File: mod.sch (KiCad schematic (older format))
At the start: 17 parts, among them IC1 ATTINY85-S, J1 MICROUSB, P1 CONN_12, Q2 FDD8870, SW1 SW_PUSH_SMALL, SW2 SW_PUSH_SMALL, SW3 SW_PUSH_SMALL

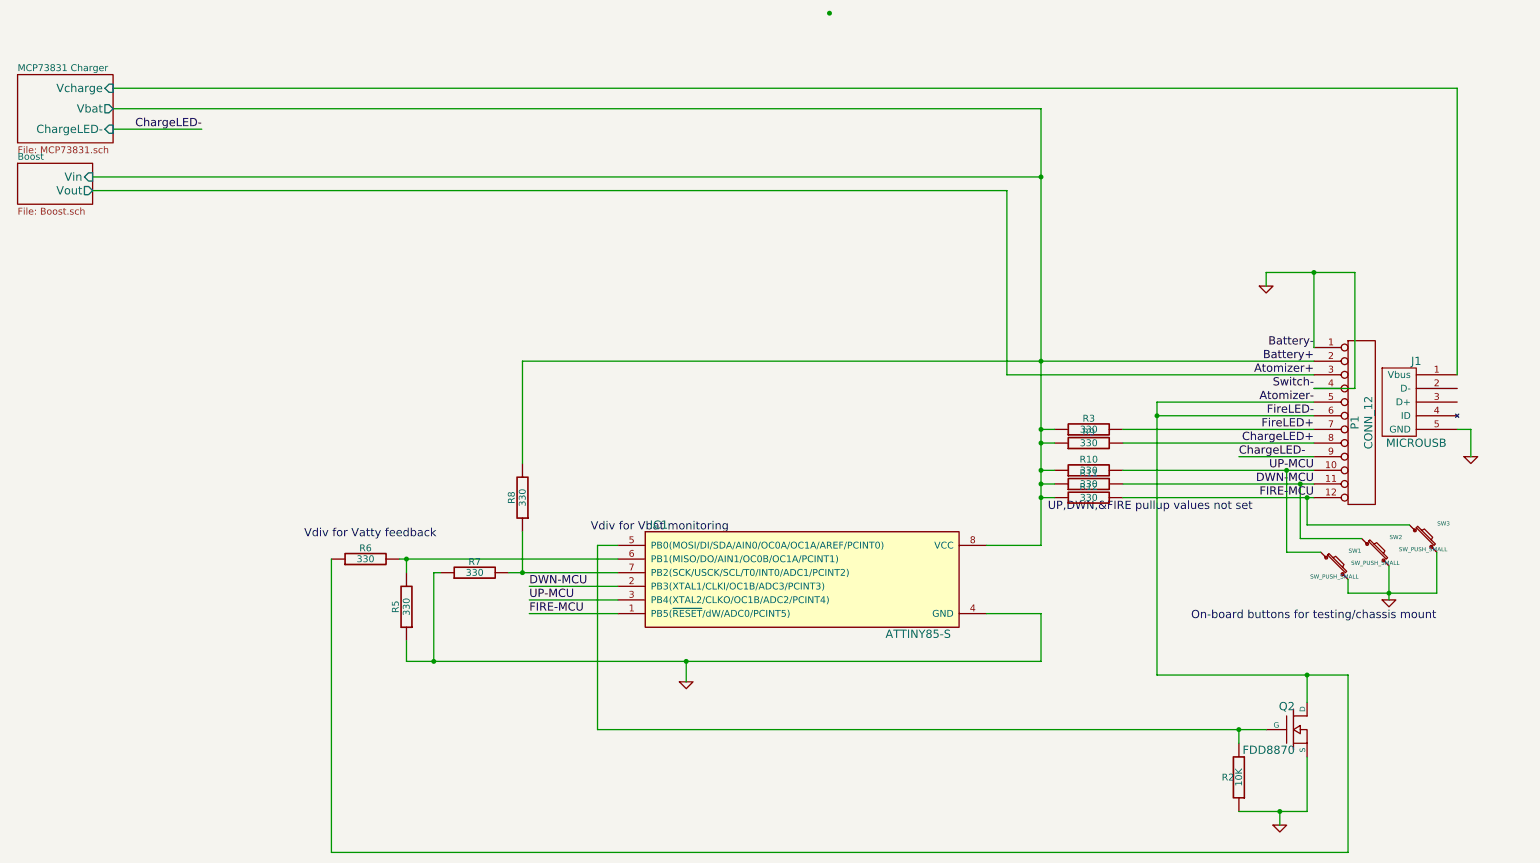
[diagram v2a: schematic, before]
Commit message: many changes. Most not stable. Check TODO
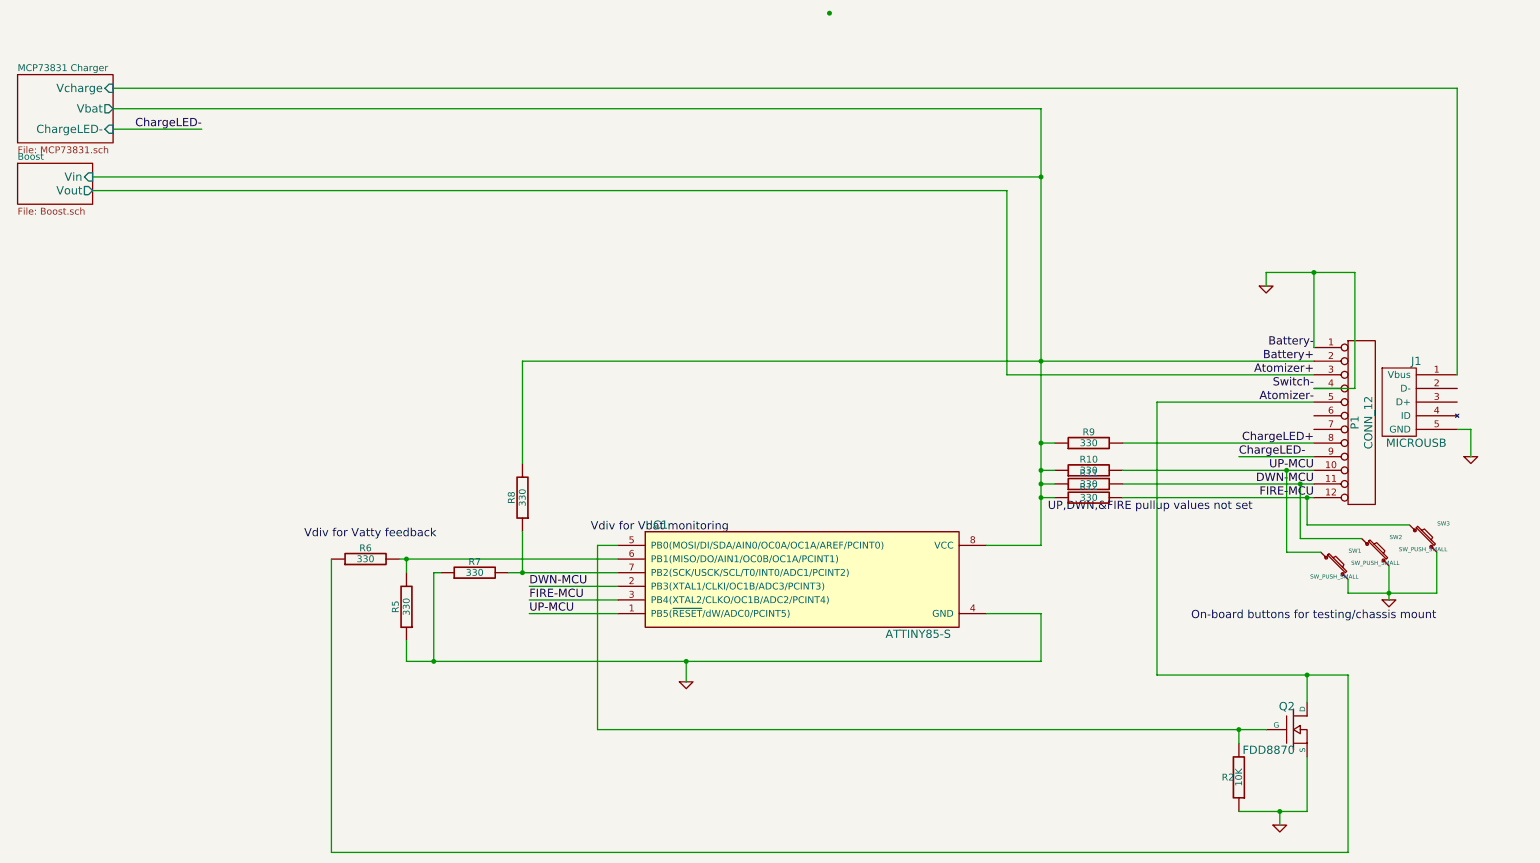
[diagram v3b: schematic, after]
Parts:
- removed R3: 330, symbol R
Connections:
- net Atomizer-: no longer P1.6 (P6)
- net FIRE-MCU: now also IC1.3 (PB4(XTAL2/CLKO/OC1B/ADC2/PCINT4)); no longer IC1.1 (PB5(~RESET~/dW/ADC0/PCINT5))
- net UP-MCU: now also IC1.1 (PB5(~RESET~/dW/ADC0/PCINT5)); no longer IC1.3 (PB4(XTAL2/CLKO/OC1B/ADC2/PCINT4))
- net FireLED+: no longer names the net of P1.7 (P7)
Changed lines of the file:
@@
-EESchema Schematic File Version 2  date Fri 29 Mar 2013 11:41:29 PM CDT
+EESchema Schematic File Version 2  date Sat 30 Mar 2013 02:51:58 PM CDT
 LIBS:power
 LIBS:device
@@
 $EndDescr
 $Comp
-L R R3
-U 1 1 5133879A
-P 8400 3600
-F 0 "R3" V 8480 3600 50  0000 C CNN
-F 1 "330" V 8400 3600 50  0000 C CNN
-F 2 "" H 8400 3600 60  0001 C CNN
-F 3 "" H 8400 3600 60  0001 C CNN
-	1    8400 3600
-	0    -1   -1   0
-$EndComp
-$Comp
 L R R2
 U 1 1 5131879B
@@
 	1    0    0    -1
 $EndComp
-Text Label 10050 3600 2    60   ~ 0
-FireLED+
-Text Label 10050 3500 2    60   ~ 0
-FireLED-
 $Sheet
 S 550  1000 700  500
@@
 	10050 2450 10050 3000
 Wire Wire Line
-	4250 3100 8050 3100
-Wire Wire Line
-	8050 3100 10050 3100
+	4250 3100 10050 3100
 Wire Wire Line
 	11100 3600 11200 3600
@@
 	11200 3600 11200 3800
 Wire Wire Line
-	8900 3400 8900 3500
-Wire Wire Line
-	8900 3500 8900 5400
-Wire Wire Line
-	8900 5400 10000 5400
-Wire Wire Line
-	10000 5400 10300 5400
+	8900 3400 8900 5400
+Wire Wire Line
+	8900 5400 10300 5400
 Wire Wire Line
 	10000 5400 10000 5600
 Wire Wire Line
-	8650 3600 10050 3600
-Wire Wire Line
 	8900 3400 10050 3400
-Wire Wire Line
-	8900 3500 10050 3500
-Connection ~ 8900 3500
 Connection ~ 6500 550
 Wire Wire Line
 	10000 6400 10000 6000
 Wire Wire Line
-	9500 6400 9800 6400
-Wire Wire Line
-	9800 6400 10000 6400
+	9500 6400 10000 6400
 Wire Wire Line
 	9800 6400 9800 6500
@@
 Connection ~ 8050 3100
 Wire Wire Line
-	9700 2450 10050 2450
-Wire Wire Line
-	10050 2450 10350 2450
+	9700 2450 10350 2450
 Wire Wire Line
 	9700 2450 9700 2550
@@
 	5450 5300 5450 5450
 Wire Wire Line
-	3400 5300 3600 5300
-Wire Wire Line
-	3600 5300 5450 5300
-Wire Wire Line
-	5450 5300 8050 5300
+	3400 5300 8050 5300
 Connection ~ 5450 5300
 Wire Wire Line
@@
 	2850 4550 2850 6700
 Wire Wire Line
-	3350 4550 3400 4550
-Wire Wire Line
-	3400 4550 4950 4550
+	3350 4550 4950 4550
 Wire Wire Line
 	3400 5150 3400 5300
 Wire Wire Line
-	4800 5800 9500 5800
-Wire Wire Line
-	9500 5800 9700 5800
+	4800 5800 9700 5800
 Wire Wire Line
 	9500 5900 9500 5800
@@
 Connection ~ 10050 2450
 Wire Wire Line
-	4150 4650 4250 4650
-Wire Wire Line
-	4250 4650 4950 4650
+	4150 4650 4950 4650
 Connection ~ 4250 4650
 Wire Wire Line
-	8650 4100 10000 4100
-Wire Wire Line
-	10000 4100 10050 4100
+	8650 4100 10050 4100
 Wire Wire Line
 	3650 4650 3600 4650
@@
 Connection ~ 8050 4100
 Wire Wire Line
-	8650 4000 9950 4000
-Wire Wire Line
-	9950 4000 10050 4000
-Wire Wire Line
-	8650 3900 9850 3900
-Wire Wire Line
-	9850 3900 10050 3900
-Wire Wire Line
-	8050 1250 8050 1750
-Wire Wire Line
-	8050 1750 8050 3100
-Wire Wire Line
-	8050 3100 8050 3600
-Wire Wire Line
-	8050 3600 8050 3700
-Wire Wire Line
-	8050 3700 8050 3900
-Wire Wire Line
-	8050 3900 8050 4000
-Wire Wire Line
-	8050 4000 8050 4100
-Wire Wire Line
-	8050 4100 8050 4450
-Wire Wire Line
-	8150 3600 8050 3600
-Connection ~ 8050 3600
+	8650 4000 10050 4000
+Wire Wire Line
+	8650 3900 10050 3900
+Wire Wire Line
+	8050 1250 8050 4450
+Wire Wire Line
+	4950 4950 4300 4950
+Wire Wire Line
+	4950 4750 4300 4750
 Wire Wire Line
 	4950 4850 4300 4850
-Wire Wire Line
-	4950 4750 4300 4750
-Wire Wire Line
-	4950 4950 4300 4950
 Wire Wire Line
 	10000 4300 10000 4100
@@
 	9850 4500 9850 3900
 Connection ~ 9850 3900
-Text Label 4300 4850 0    60   ~ 0
+Text Label 4300 4950 0    60   ~ 0
 UP-MCU
 Text Label 4300 4750 0    60   ~ 0
 DWN-MCU
-Text Label 4300 4950 0    60   ~ 0
+Text Label 4300 4850 0    60   ~ 0
 FIRE-MCU
 Wire Wire Line
@@
 $EndComp
 Wire Wire Line
-	10600 4600 10600 4800
-Wire Wire Line
-	10600 4800 10600 4850
+	10600 4600 10600 4850
 Wire Wire Line
 	10300 4700 10300 4800
 Wire Wire Line
-	10300 4800 10600 4800
-Wire Wire Line
-	10600 4800 10950 4800
+	10300 4800 10950 4800
 Connection ~ 10600 4800
 Wire Wire Line

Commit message: morning updates
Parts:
- removed J1: MICROUSB, symbol MICROUSB
- removed Q2: FDD8870, symbol MOSFET_N
- removed R2: 10K, symbol R
- removed R9: 330, symbol R
- P2: renamed from P1; symbol CONN_12 -> CONN_10
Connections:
- net ChargeLED+ is gone; now on net UP-MCU: P2.8 (P8)
- net ChargeLED- is gone; now on net DWN-MCU: P2.9 (P9)
- net Atomizer-: now also P2.4 (P4); no longer P2.5 (P5)
- net DWN-MCU: no longer P2.11 (P11)
- net FIRE-MCU: now also P2.10 (P10); no longer P2.12 (P12)
- net GND: no longer P2.4 (P4)
- net UP-MCU: no longer P2.10 (P10)
- net Simple PCB/GATE: now reaches IC1.5 (PB0(MOSI/DI/SDA/AIN0/OC0A/OC1A/AREF/PCINT0))
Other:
- note added: "Vdiv resistor values not yet set!"
- moved on the sheet: R10, R11, R12, R8
